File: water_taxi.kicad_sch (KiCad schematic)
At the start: 19 parts

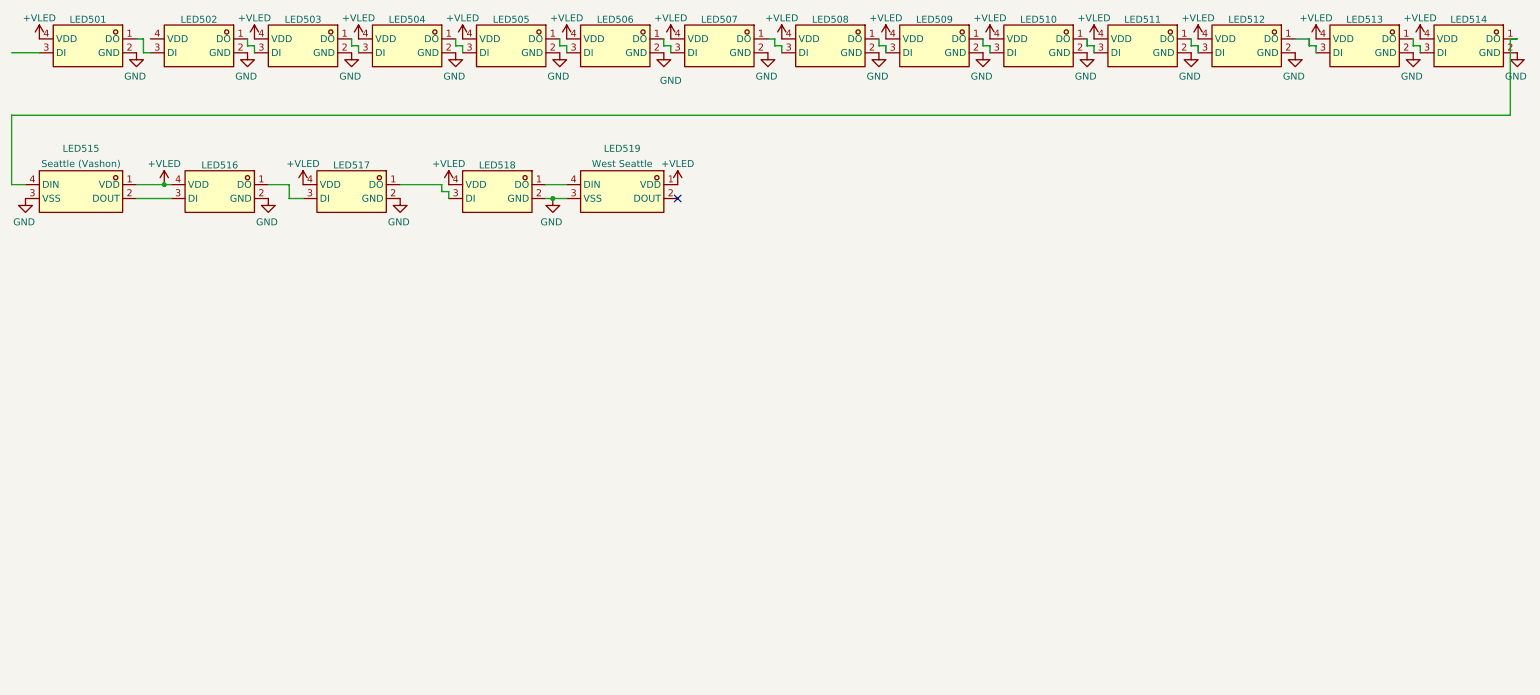
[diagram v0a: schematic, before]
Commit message: junction checkpoint
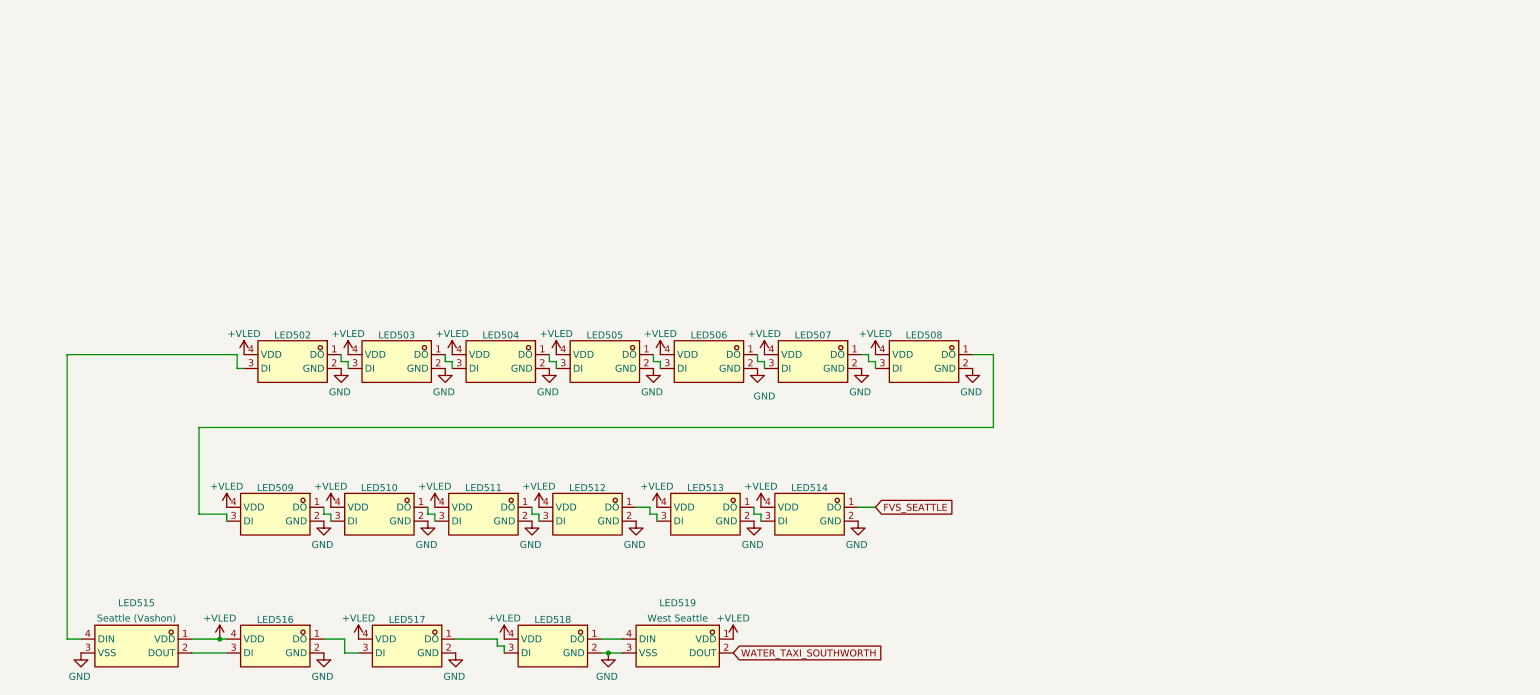
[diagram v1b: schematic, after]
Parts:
- removed LED501: WS2812B-2020, EasyEDA:LED-SMD_4P-L2.0-W2.0-TL_WS2812B-2020, symbol EasyEDA:WS2812B-2020
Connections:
- net +VLED: now also LED502.4 (VDD)
- net at LED515.4 (DIN): now also LED502.3 (DI); no longer LED514.1 (DO)
- net WATER_TAXI_SOUTHWORTH: now reaches LED519.2 (DOUT)
- new net FVS_SEATTLE: LED514.1 (DO)
- no-connect marks 1 -> 0
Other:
- moved on the sheet: LED502, LED503, LED504, LED505, LED506, LED507, LED508, LED509, LED510, LED511, LED512, LED513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
